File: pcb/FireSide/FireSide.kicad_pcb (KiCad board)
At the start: 2 copper layers, 120 x 80 mm, 27 parts, among them J0 SDIOModule, J1 D4184_PIN_A, J10 5V_01x02_JST, J11 5V_01x02_JST, J12 Status_01x02_JST, J2 D4184_PIN_B, J3 D4184_PIN_C, J4 A0_01x02_JST, J5 A1_01x02_JST, J6 A2_01x02_JST, J60 XT60-Male, J7 A3_01x02_JST, J8 A4_01x02_JST, J9 A5_01x02_JST, Q1 MMBT2222A, U1 AMS1117-5.0, U3 RYLR998

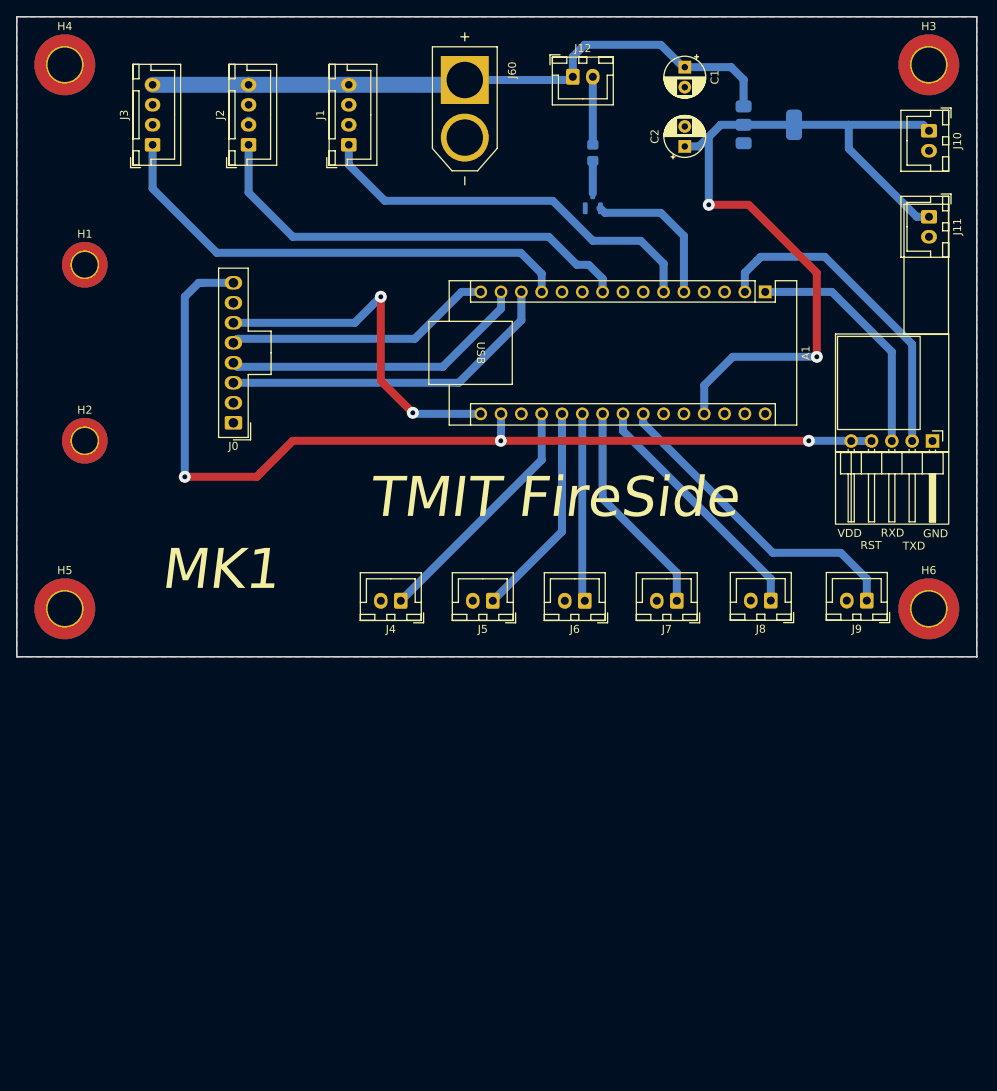
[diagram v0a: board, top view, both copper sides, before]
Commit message: [FS] PCB Updated to v1.1.6
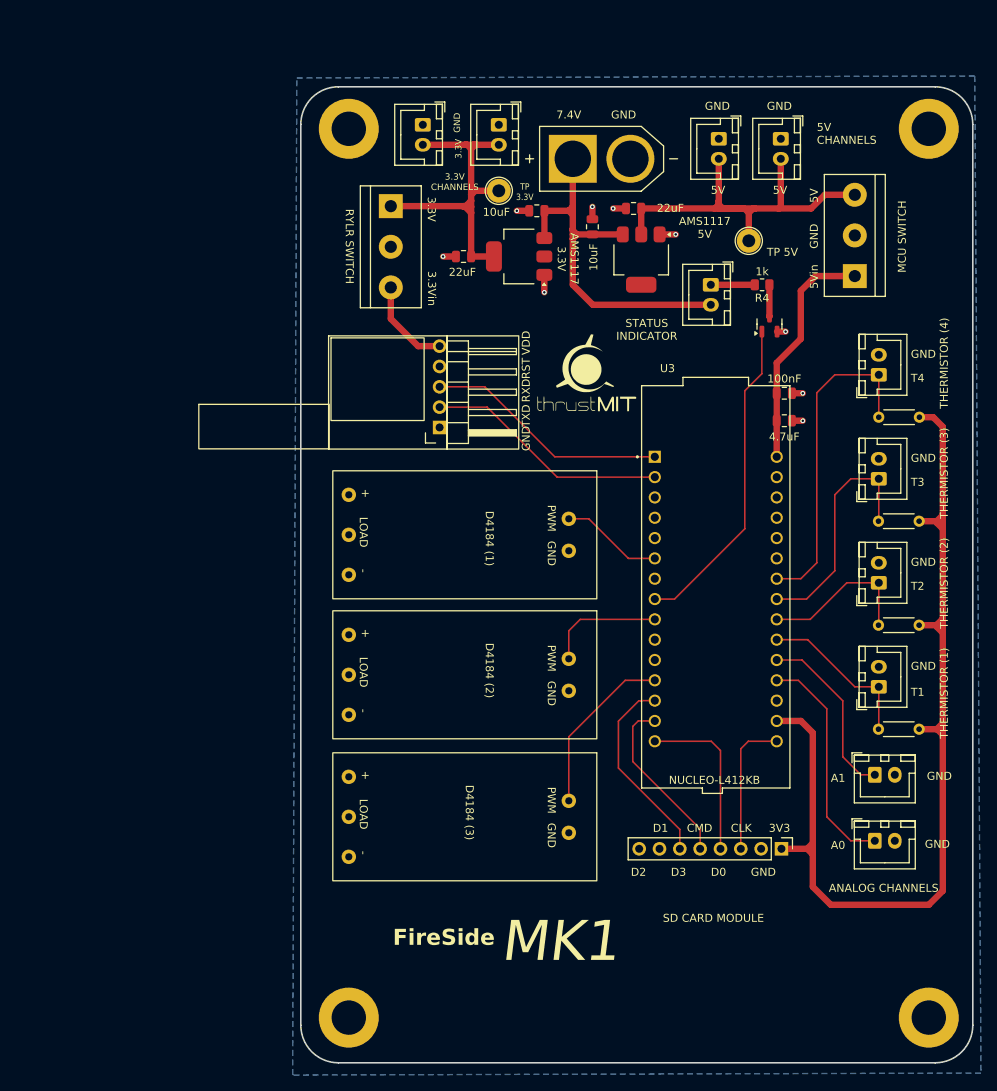
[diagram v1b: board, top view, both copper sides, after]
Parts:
- removed A1: Nucleo-L412KB, Module:Arduino_Nano
- removed H5, H6: BoardM4, MountingHole:MountingHole_4.3mm_M4_ISO7380_Pad_TopBottom
- removed J0: SDIOModule, Connector_Molex:Molex_Nano-Fit_105309-xx08_1x08_P2.50mm_Vertical
- removed J60: XT60-Male, XT60-M:AMASS_XT60-M
- removed R1: 1k, Resistor_SMD:R_0805_2012Metric_Pad1.20x1.40mm_HandSolder
- added C3: 10uF, Capacitor_SMD:C_0805_2012Metric, F.Cu at (107.0, 46.8)
- added C4: 22uF, Capacitor_SMD:C_0805_2012Metric, F.Cu at (90.8, 50.5)
- added C5: 100nF, Capacitor_SMD:C_0805_2012Metric, F.Cu at (130.9, 67.6)
- added C6: 4.7uF, Capacitor_SMD:C_0805_2012Metric, F.Cu at (130.9, 71.0)
- added G***: LOGO, logos:logo2, F.Cu at (106.1, 64.4)
- added J13: Screw_Terminal_01x03, TerminalBlock:TerminalBlock_bornier-3_P5.08mm, F.Cu at (139.8, 52.9)
- added J14: Conn_01x02_Pin, Connector_JST:JST_XH_B2B-XH-A_1x02_P2.50mm_Vertical, F.Cu at (142.8, 65.2)
- added R2: 100k, Resistor_THT:R_Axial_DIN0204_L3.6mm_D1.6mm_P5.08mm_Horizontal, F.Cu at (147.8, 109.5)
- added R4: 1k, Resistor_SMD:R_0805_2012Metric, F.Cu at (128.2, 54.0)
- added R5: 100k, Resistor_THT:R_Axial_DIN0204_L3.6mm_D1.6mm_P5.08mm_Horizontal, F.Cu at (147.8, 96.5)
- added R6: 100k, Resistor_THT:R_Axial_DIN0204_L3.6mm_D1.6mm_P5.08mm_Horizontal, F.Cu at (147.8, 83.5)
- added R7: 100k, Resistor_THT:R_Axial_DIN0204_L3.6mm_D1.6mm_P5.08mm_Horizontal, F.Cu at (147.8, 70.5)
- added TP1: TestPoint, TestPoint:TestPoint_Loop_D2.60mm_Drill1.6mm_Beaded, F.Cu at (126.5, 48.5)
- added TP2: TestPoint, TestPoint:TestPoint_Loop_D2.60mm_Drill1.6mm_Beaded, F.Cu at (95.2, 42.2)
- added U2: ~, FireSide Footprint:RYLR998, F.Cu at (78.7, 67.3)
- added U4: AMS1117-5.0, Package_TO_SOT_SMD:SOT-223-3_TabPin2, F.Cu at (113.0, 50.9)
- added U5: ~, FireSide Footprint:D4184, F.Cu at (95.0, 85.8)
- added U6: ~, FireSide Footprint:D4184, F.Cu at (95.0, 121.0)
- added U8: ~, FireSide Footprint:XT60-M, F.Cu at (107.6, 29.6)
- added U9: ~, FireSide Footprint:D4184, F.Cu at (95.0, 103.2)
- C1: value 22u -> 22uF; footprint Capacitor_THT:CP_Radial_D5.0mm_P2.50mm -> Capacitor_SMD:C_0805_2012Metric
- C2: value 22u -> 10uF; footprint Capacitor_THT:CP_Radial_D5.0mm_P2.50mm -> Capacitor_SMD:C_0805_2012Metric
- H1, H2: value SDModuleM3 -> MountingHole_Pad; footprint MountingHole:MountingHole_3.2mm_M3_ISO7380_Pad_TopBottom -> MountingHole:MountingHole_4.3mm_M4_DIN965_Pad
- H3, H4: value BoardM4 -> MountingHole_Pad; footprint MountingHole:MountingHole_4.3mm_M4_ISO7380_Pad_TopBottom -> MountingHole:MountingHole_4.3mm_M4_DIN965_Pad
- J1: value D4184_PIN_A -> Conn_01x02_Pin; footprint Connector_JST:JST_XH_B4B-XH-A_1x04_P2.50mm_Vertical -> Connector_JST:JST_XH_B2B-XH-A_1x02_P2.50mm_Vertical
- J10, J11: value 5V_01x02_JST -> Conn_01x02_Pin
- J12: value Status_01x02_JST -> Conn_01x02_Pin
- J2: value D4184_PIN_B -> Conn_01x02_Pin; footprint Connector_JST:JST_XH_B4B-XH-A_1x04_P2.50mm_Vertical -> Connector_JST:JST_XH_B2B-XH-A_1x02_P2.50mm_Vertical
- J3: value D4184_PIN_C -> Conn_01x08_Pin; footprint Connector_JST:JST_XH_B4B-XH-A_1x04_P2.50mm_Vertical -> Connector_PinHeader_2.54mm:PinHeader_1x08_P2.54mm_Vertical
- J4: value A0_01x02_JST -> Conn_01x02_Pin
- J5: value A1_01x02_JST -> Conn_01x02_Pin
- J6: value A2_01x02_JST -> Conn_01x02_Pin
- J7: value A3_01x02_JST -> Conn_01x02_Pin
- J8: value A4_01x02_JST -> Conn_01x02_Pin
- J9: value A5_01x02_JST -> Screw_Terminal_01x03; footprint Connector_JST:JST_XH_B2B-XH-A_1x02_P2.50mm_Vertical -> TerminalBlock:TerminalBlock_bornier-3_P5.08mm
- Q1: moved to F.Cu
- U1: value AMS1117-5.0 -> AMS1117-3.3; moved to F.Cu
- U3: value RYLR998 -> NUCLEO-L412KB; footprint RYLR998:RYLR998 -> FireSide Footprint:NUCLEO-L412KB
- moved H1 141.4 mm to (149.0, 145.6), turned to 90 degrees
- moved J3 118.0 mm to (130.6, 124.5), turned to -90 degrees
- moved J2 111.0 mm to (142.2, 115.2), turned to 0 degrees
- moved J1 109.1 mm to (142.2, 123.5), turned to 0 degrees
- moved H4 108.3 mm to (149.0, 34.5), turned to 90 degrees
- moved H2 79.3 mm to (76.5, 145.6), turned to 90 degrees
- moved J9 77.3 mm to (81.8, 44.2), turned to -90 degrees
- moved H3 72.9 mm to (76.5, 34.5), turned to 90 degrees
- moved J11 64.3 mm to (85.8, 34.0)
- moved J4 60.7 mm to (142.8, 104.2), turned to 90 degrees
- moved J7 58.0 mm to (122.8, 35.8), turned to -90 degrees
- moved J8 57.7 mm to (130.5, 35.8), turned to -90 degrees
- moved J5 48.3 mm to (142.8, 91.2), turned to 90 degrees
- moved J6 39.8 mm to (142.8, 78.2), turned to 90 degrees
- moved U1 35.3 mm to (97.8, 50.5), turned to 180 degrees
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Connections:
- C1 pad 1: +BATT -> 5V
- C2 pad 1: /5VIN -> VI
- J1 pad 1: /FIRE_PIN_A -> A0
- J10 pad 1: /5VIN -> Net-(J10-Pin_1)
- J10 pad 2: GND -> VI
- J11 pad 1: /5VIN -> GND
- J11 pad 2: GND -> 3.3V
- J12 pad 1: +BATT -> GND
- J12 pad 2: Net-(J12-Pin_2) -> 3.3V
- J2 pad 1: /FIRE_PIN_B -> A1
- J3 pad 1: /FIRE_PIN_C -> 3.3V_STM
- J3 pad 3: GND -> SCK_SD
- J3 pad 4: +BATT -> MISO_SD
- J4 pad 1: Net-(A1-A0) -> A_THERM-1
- J5 pad 1: Net-(A1-A1) -> A_THERM-2
- J6 pad 1: Net-(A1-A2) -> A_THERM-3
- J7 pad 1: Net-(A1-A3) -> GND
- J7 pad 2: GND -> 5V
- J8 pad 1: Net-(A1-SDA/A4) -> GND
- J8 pad 2: GND -> 5V
- J9 pad 1: Net-(A1-SCL/A5) -> 3.3V
- Q1 pad 1: /STATUS_PIN -> STATUS_PIN
- U1 pad 2: /5VIN -> 3.3V
- U1 pad 3: +BATT -> VI
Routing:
- net 3.3V_STM: track 0.00 -> 125.6 mm
- net Net-(A1-3V3): track 120.4 -> 0.00 mm, vias 3 -> 0
- net /5VIN: track 103.6 -> 0.00 mm, vias 2 -> 0
- net +BATT: track 82.6 -> 0.00 mm
- net /FIRE_PIN_C: track 60.8 -> 0.00 mm
- net /FIRE_PIN_B: track 56.3 -> 0.00 mm
- net 5V: track 0.00 -> 53.0 mm
- net VI: track 0.00 -> 50.8 mm
- net /FIRE_PIN_A: track 50.5 -> 0.00 mm
- net 3.3V: track 0.00 -> 46.0 mm
- net Net-(A1-SCK): track 44.5 -> 0.00 mm, vias 2 -> 0
- net Net-(A1-D10): track 42.8 -> 0.00 mm
- net A_THERM-4: track 0.00 -> 41.1 mm
- net Net-(A1-RX1): track 40.8 -> 0.00 mm
- net STATUS_PIN: track 0.00 -> 40.4 mm
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- removed copper zone on F.Cu, net GND
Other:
- board size 120 x 80 mm -> 84 x 122 mm
- board text added: "-------------- SANYUKTA DUTTA TEJASWINEE GUNJAL KRISHNA GUND MYTREYA BADAMPUDI YASH PATIDAR RISHIT KULKARNI DEEPSHIKHA SARANGI --------------"
- board text added: "10uF"
- board text added: "22uF"
- board text added: "3.3V"
- board text added: "3.3V CHANNELS"
- board text added: "3.3Vin"
- board text added: "3V3"
- board text added: "5V"
- board text added: "5V CHANNELS"
- board text added: "5Vin"
- board text added: "7.4V"
- board text added: "A0"
- board text added: "A1"
- board text added: "AMS1117 3.3V"
- board text added: "AMS1117 5V"
- board text added: "ANALOG CHANNELS"
- board text added: "CLK"
- board text added: "CMD"
- board text added: "D0"
- board text added: "D0-TX_RYLR D1-RX_RYLR D2-LAUNCH_LED D4-ARM_LED D3-D4184(1) D6-D4184(2) D9-D4184(3) D5-STATUS D10-CS D11-MOSI D12-MISO D13-SCK A0:A1-ANALOG A2:A5-THERM"
- board text added: "D1"
- board text added: "D2"
- board text added: "D3"
- board text added: "D4184 (1)"
- board text added: "D4184 (2)"
- board text added: "D4184 (3)"
- board text added: "FireSide"
- board text added: "GND"
- board text added: "MCU SWITCH"
- board text added: "NUCLEO-L412KB"
- board text added: "RYLR SWITCH"
- board text added: "SD CARD MODULE"
- board text added: "STATUS INDICATOR"
- board text added: "T1"
- board text added: "T2"
- board text added: "T3"
- board text added: "T4"
- board text added: "THERMISTOR (1)"
- board text added: "THERMISTOR (2)"
- board text added: "THERMISTOR (3)"
- board text added: "THERMISTOR (4)"
- board text added: "TP 3.3V"
- board text added: "TP 5V"
- board text added: "are you sure??"
- board text added: "special thanks to bunty"
- board text removed: "TMIT FireSide"
